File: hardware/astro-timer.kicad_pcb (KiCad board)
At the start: 2 copper layers, 65.8 x 41.4 mm, 35 parts, among them J1 AVR-ISP-6, J2 AudioJack3, Q1 Q_NPN_BEC, Q2 Q_NPN_BEC, SW1 SW_SPST, SW2 SW_Push, SW3 SW_Push, SW4 Rotary_Encoder_Switch, U1 ATmega328P-AU, Y1 Crystal

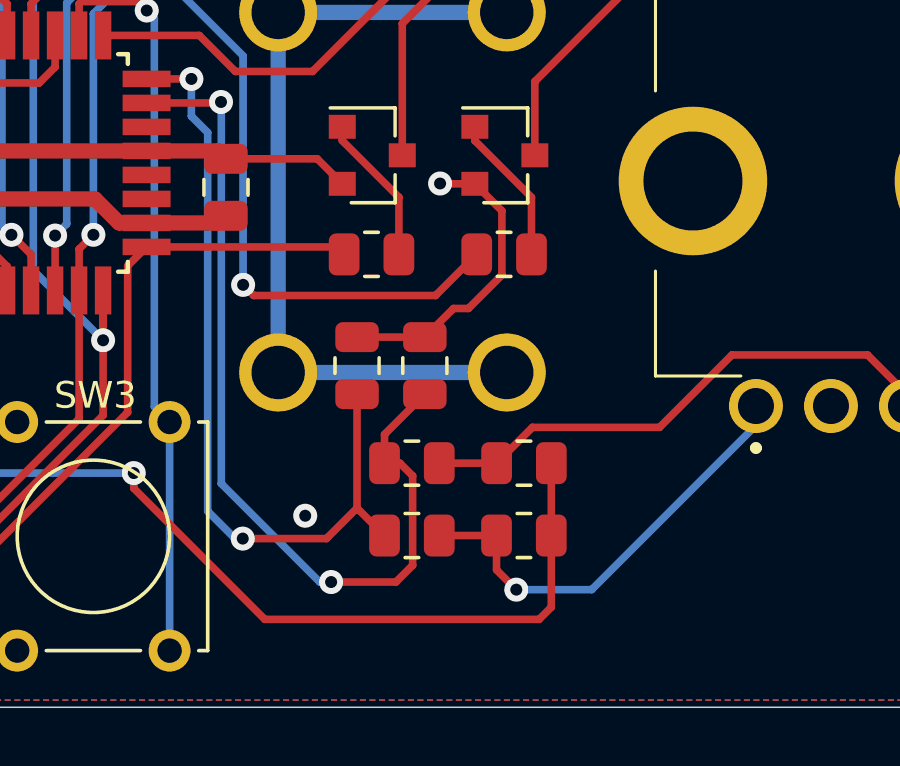
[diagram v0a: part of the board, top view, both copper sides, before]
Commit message: tweaks
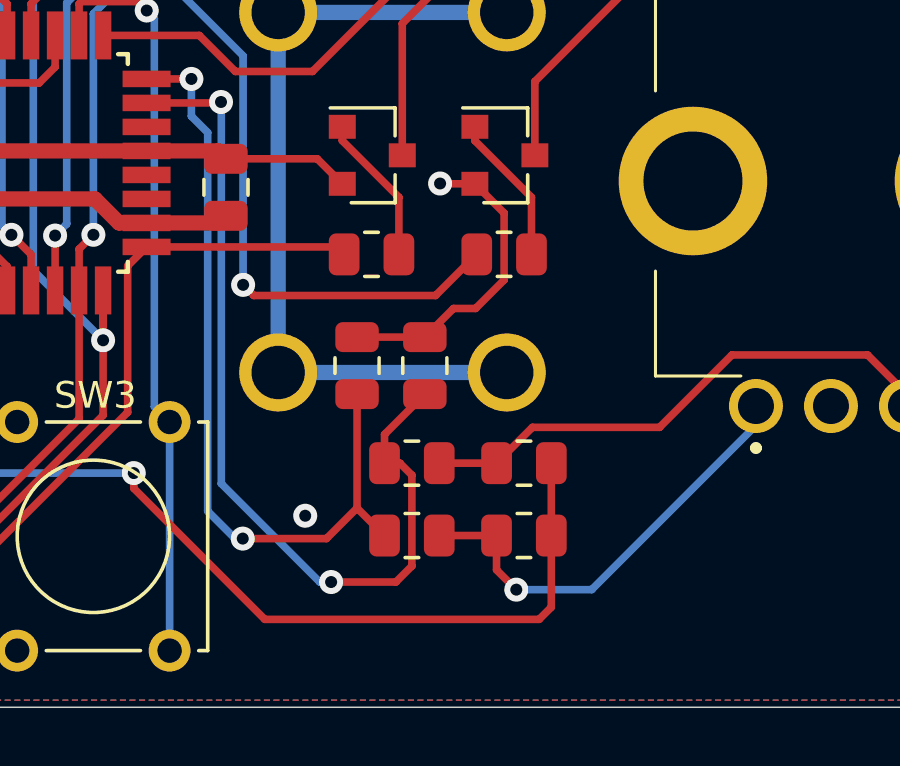
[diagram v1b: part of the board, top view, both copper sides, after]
